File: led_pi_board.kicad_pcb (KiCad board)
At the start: 2 copper layers, 65 x 30.5 mm, 32 parts, among them J1 PJ-002A, J10 Conn_02x20_Odd_Even, J11 Conn_01x04, J2 Raspberry_Pi_2_3, J3 Screw_Terminal_01x02, J4 Conn_01x25, J5 Conn_01x04, J6 Conn_01x04, J7 Conn_01x04, J8 Conn_02x08_Odd_Even, J9 Conn_01x03, U1 MAX4866LEUT-T, U2 74AHCT245, U3 74AHCT245, U4 74AHCT245, U5 ADS1015IRUGR, U6 DMC3021LSD

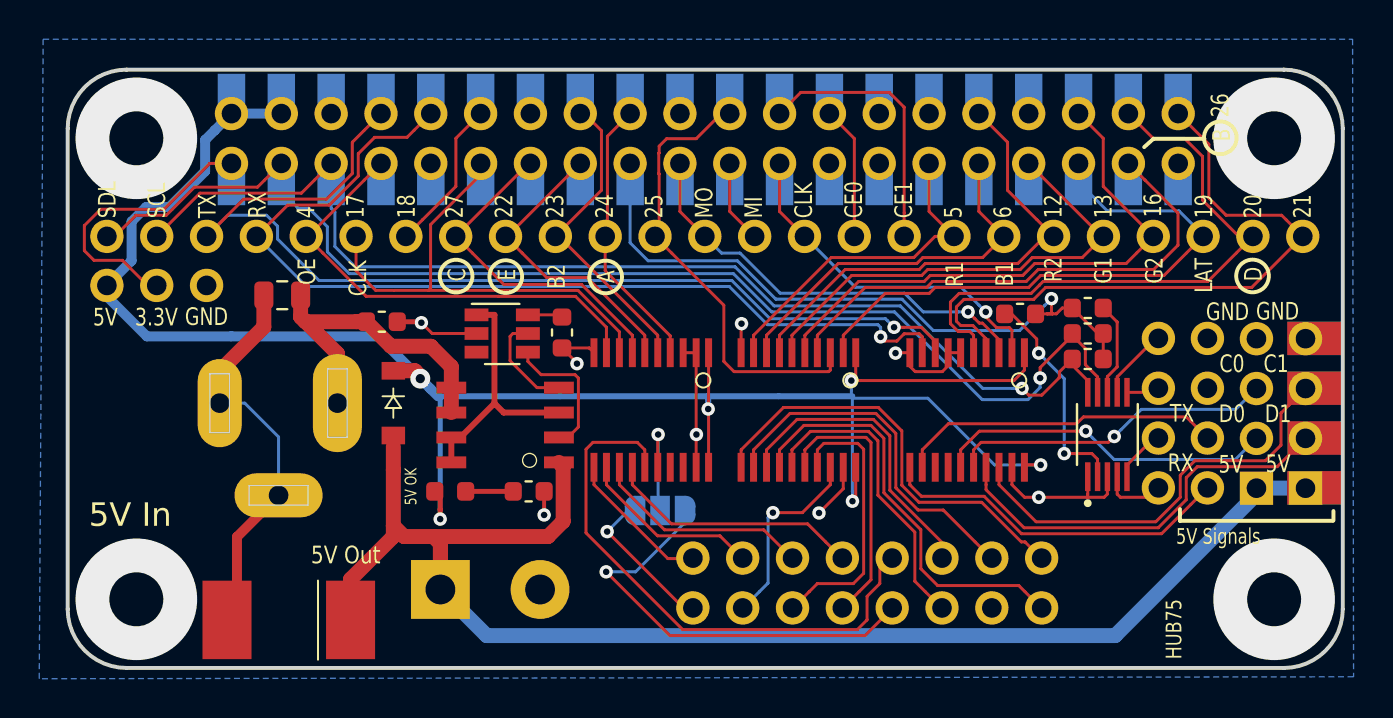
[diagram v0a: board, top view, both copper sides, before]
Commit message: version 5 updates
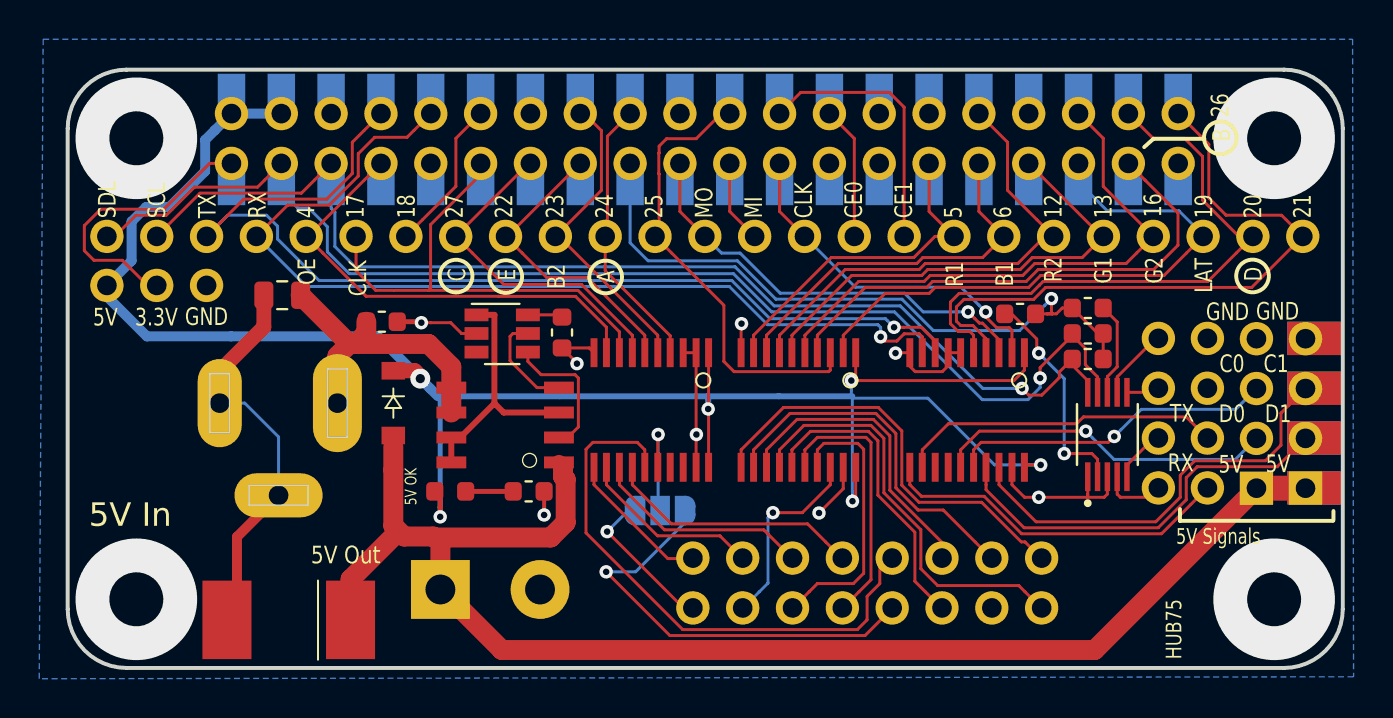
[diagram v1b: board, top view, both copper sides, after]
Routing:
- net +5VA: track 76.3 -> 79.5 mm
- net Net-(C1-Pad1): track 17.3 -> 16.5 mm
